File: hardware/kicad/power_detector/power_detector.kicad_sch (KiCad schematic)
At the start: 36 parts, among them IC1 ADL5906ACPZN-R7, IC2 ADL5906ACPZN-R7, J10 mcu_ref, J3 5v, J5 901-10511-1, J6 debug_fow, J7 debug_ref, J8 901-10511-1, J9 mcu_fwd

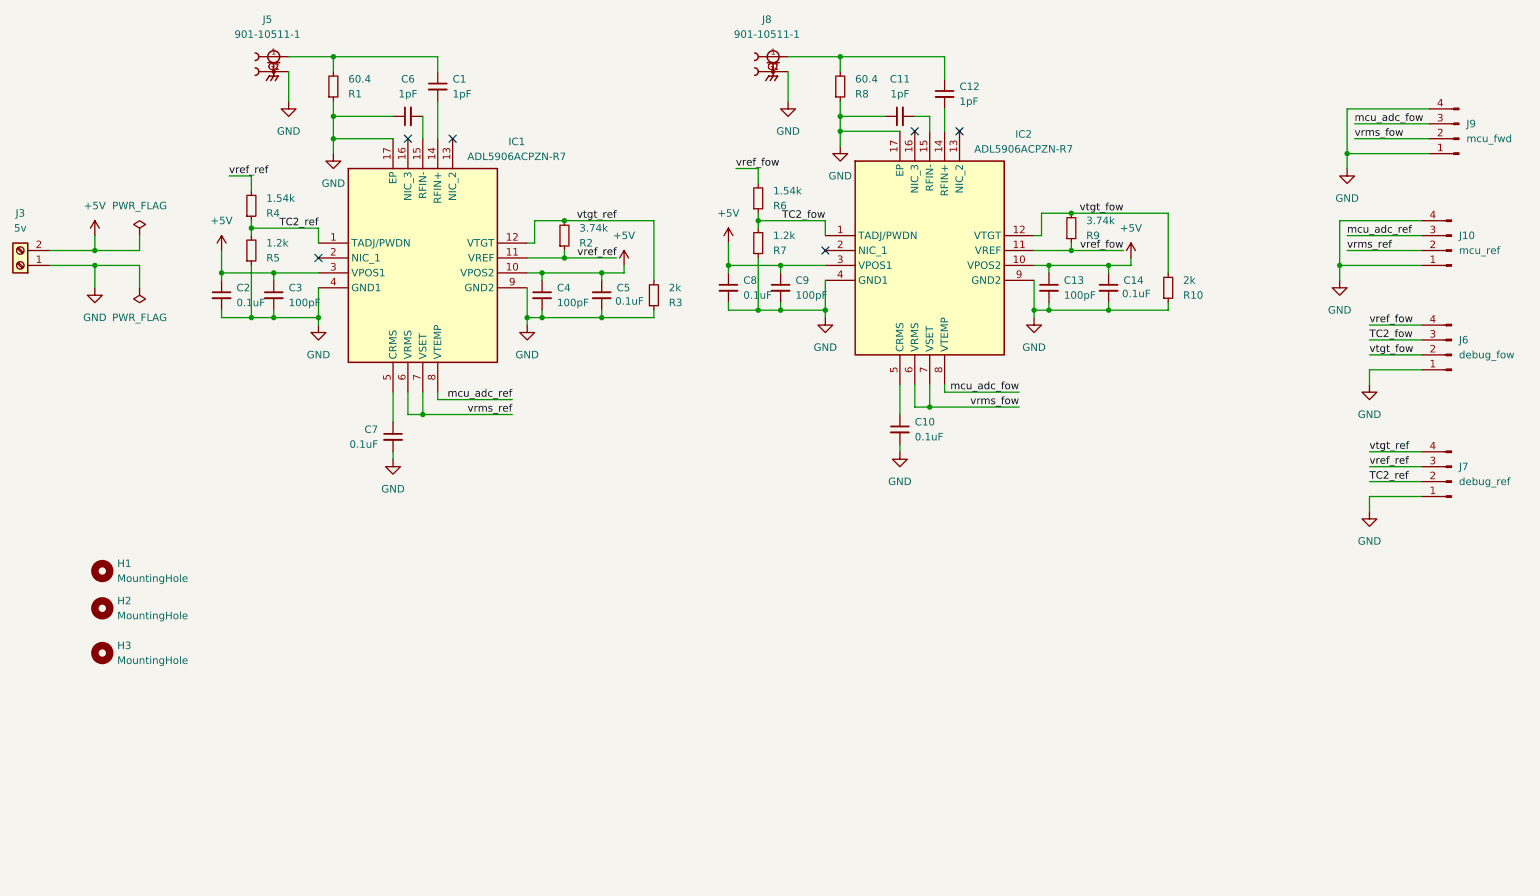
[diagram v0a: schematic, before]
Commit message: unfinished v0.5
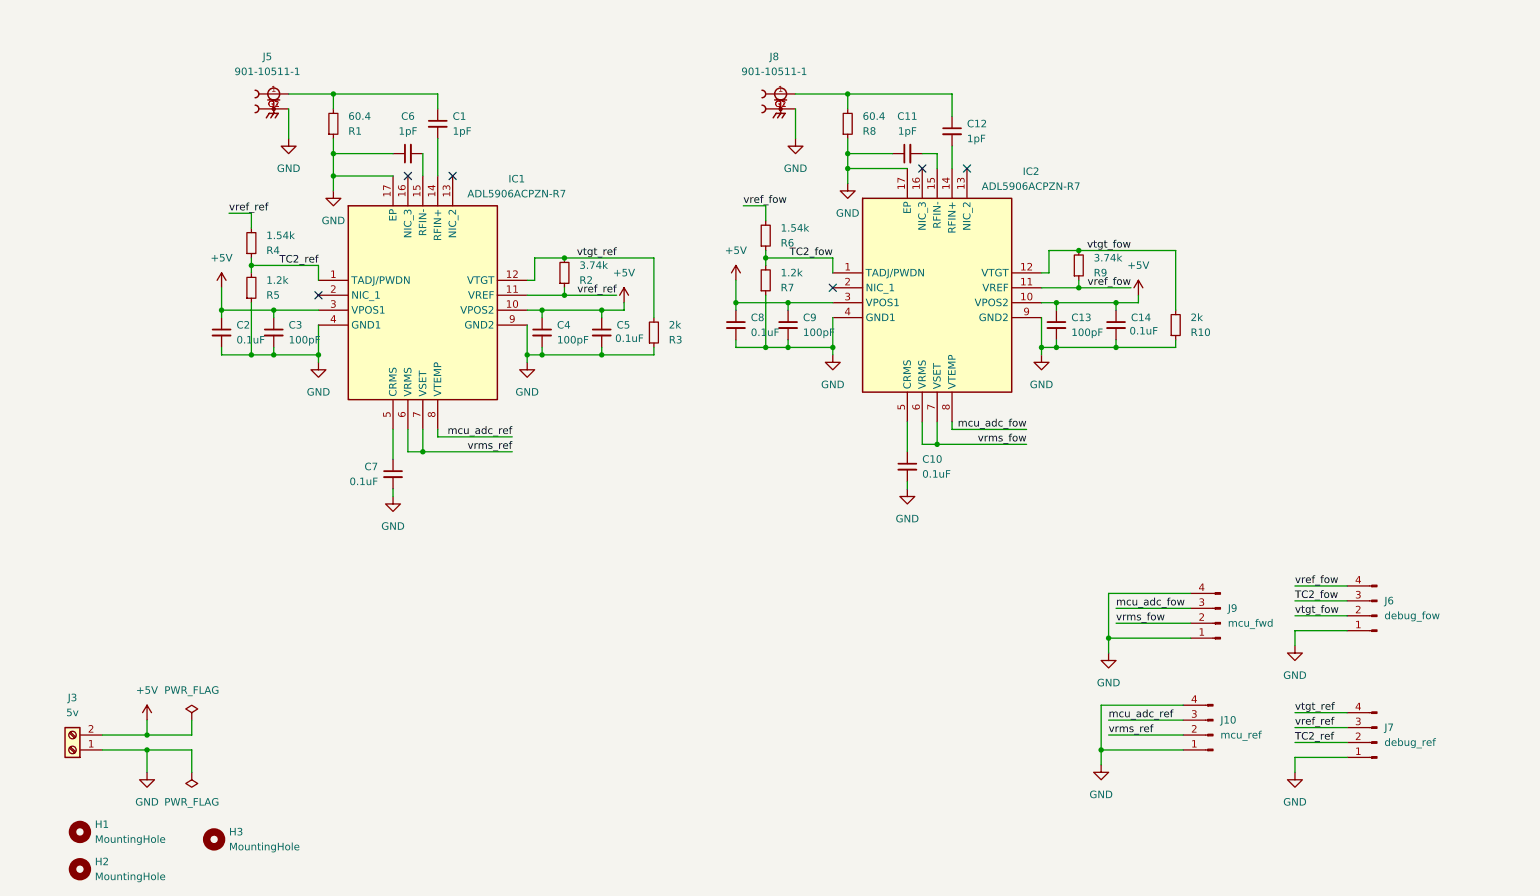
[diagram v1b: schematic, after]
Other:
- moved on the sheet: C1, C10, C11, C12, C13, C14, C2, C3, C4, C5, C6, C7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
